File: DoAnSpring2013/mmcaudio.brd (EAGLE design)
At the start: 181.9 x 121.9 mm, 84 parts, among them IC1 TL082, IC2 TL082, IC3 LM1117, IC4 TL082, IC5 TL082, U1 DAC0808LCN, U2 TEA2025B, X1 HD44780LCD-1602

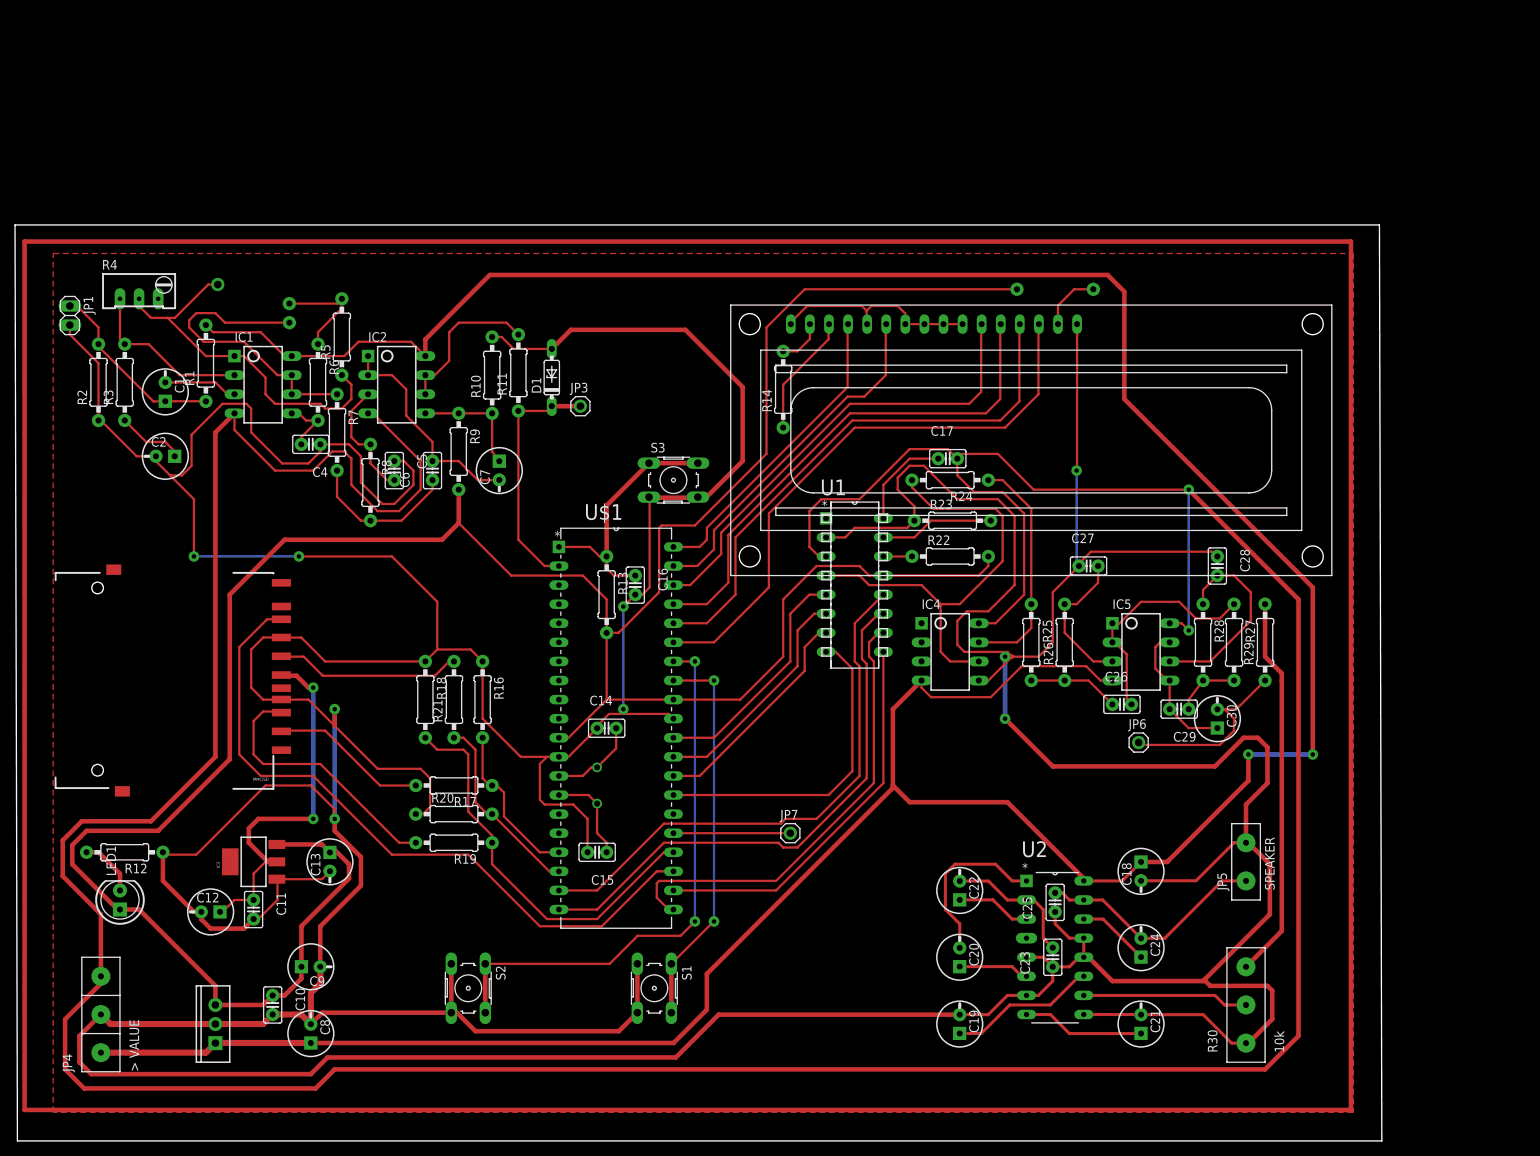
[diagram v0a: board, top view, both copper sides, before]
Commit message: notthing to update
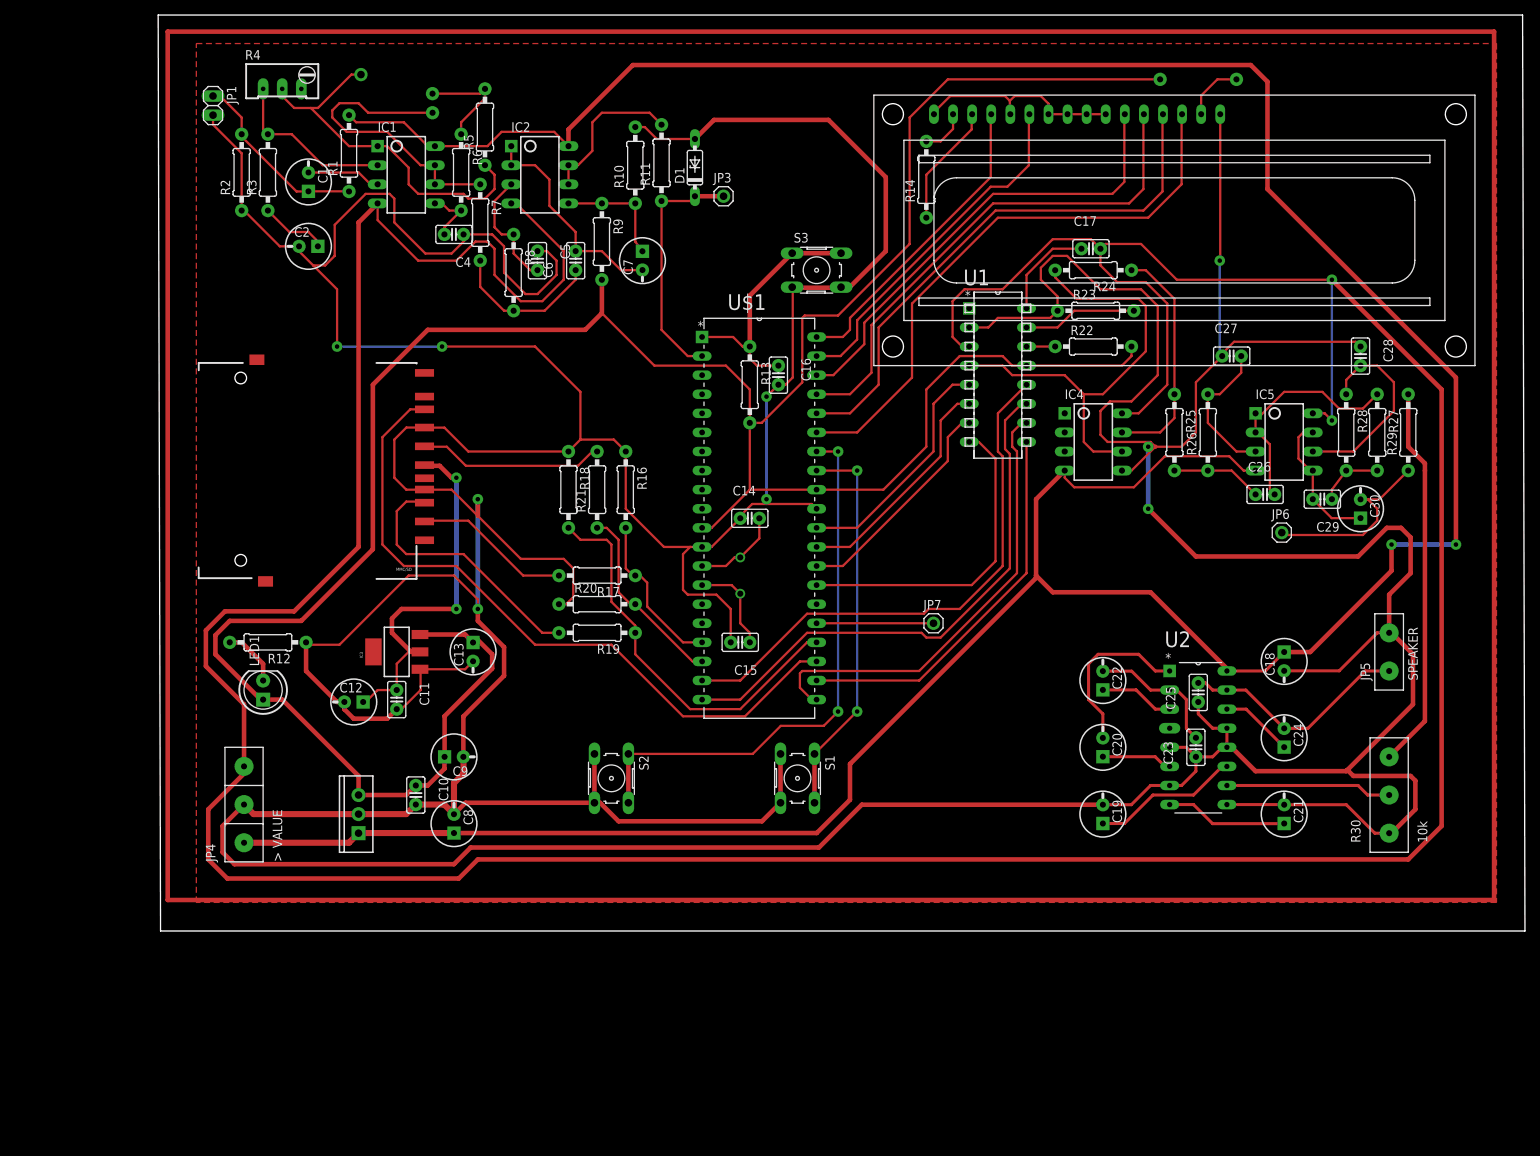
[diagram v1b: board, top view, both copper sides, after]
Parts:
- moved C27 33.8 mm to (156.8, 97.8)
- moved C28 33.8 mm to (174.0, 97.8)
- moved R5 33.8 mm to (57.5, 128.3)
- moved C14 33.8 mm to (92.7, 76.2)
- moved C24 33.8 mm to (163.8, 47.0)
- moved C25 33.8 mm to (152.4, 53.0)
- moved JP4 33.8 mm to (26.7, 33.0)
- moved LED1 33.8 mm to (27.9, 53.3)
- moved R16 33.8 mm to (76.2, 80.0)
- moved R18 33.8 mm to (68.6, 80.0)
- moved R21 33.8 mm to (72.4, 80.0)
- moved R23 33.8 mm to (138.7, 103.8)
- moved R30 33.8 mm to (177.8, 40.6)
- moved U2 33.8 mm to (156.2, 38.1)
- moved C11 33.8 mm to (45.7, 52.1)
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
